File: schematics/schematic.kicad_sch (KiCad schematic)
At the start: 14 parts, among them J2 Conn_01x02, Q1 BPW40, U1 L293D, U2 ESP32-S3-DevKitC, U3 L7805

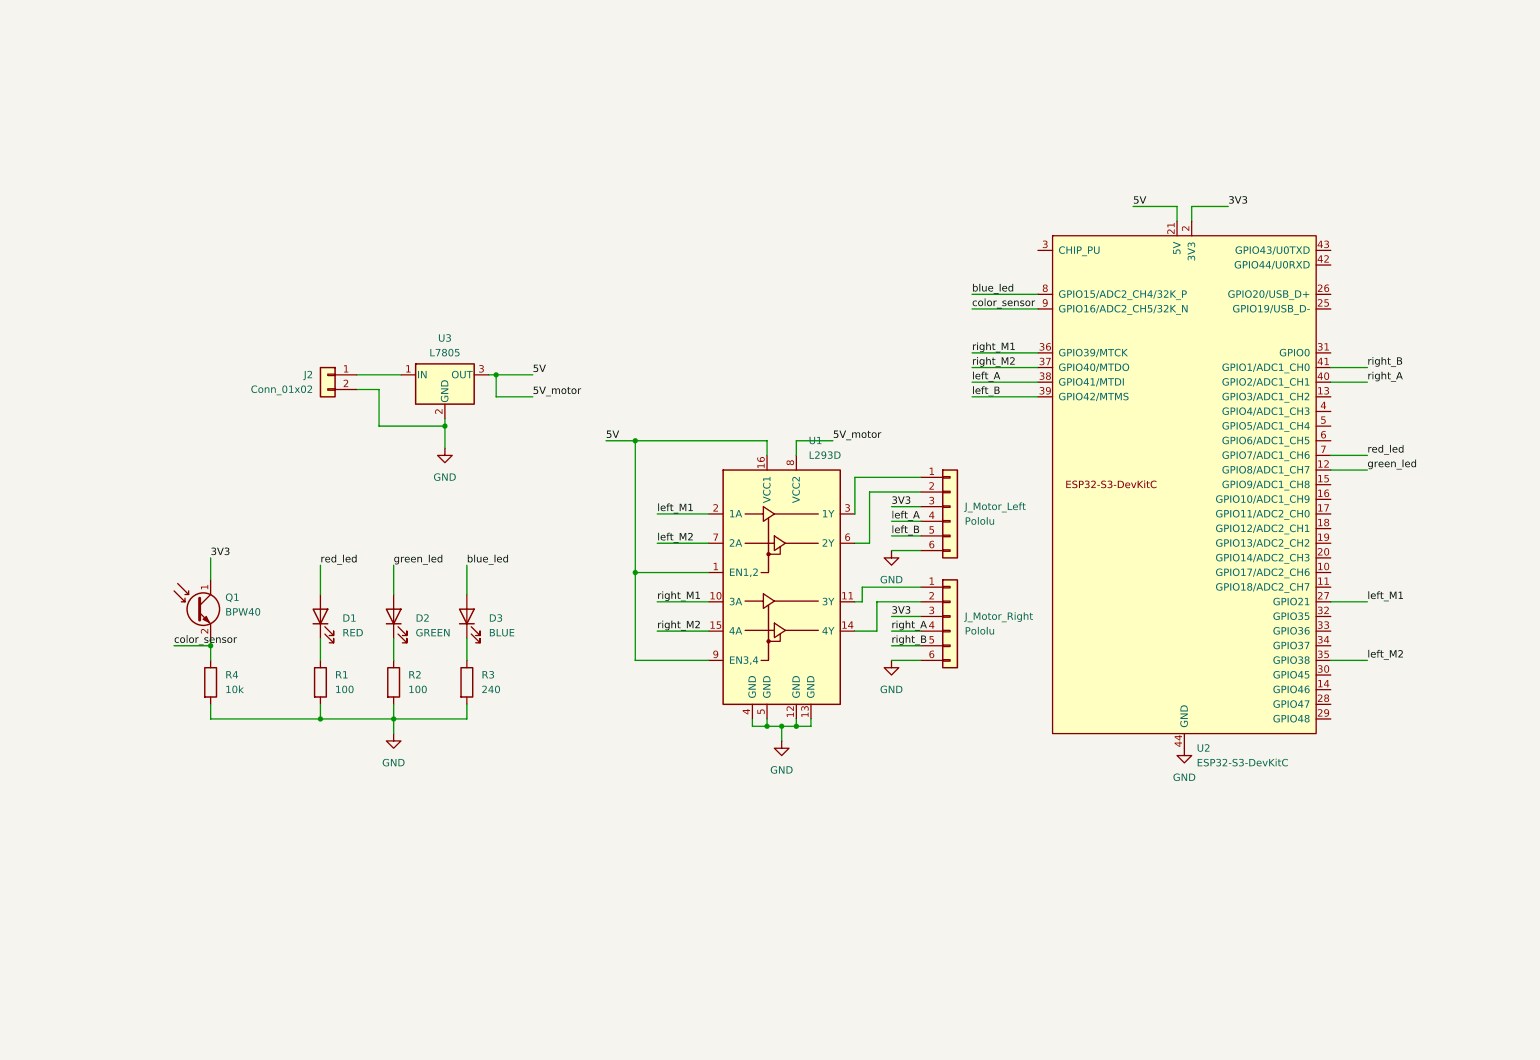
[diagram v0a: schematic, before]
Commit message: schematic update: almost done
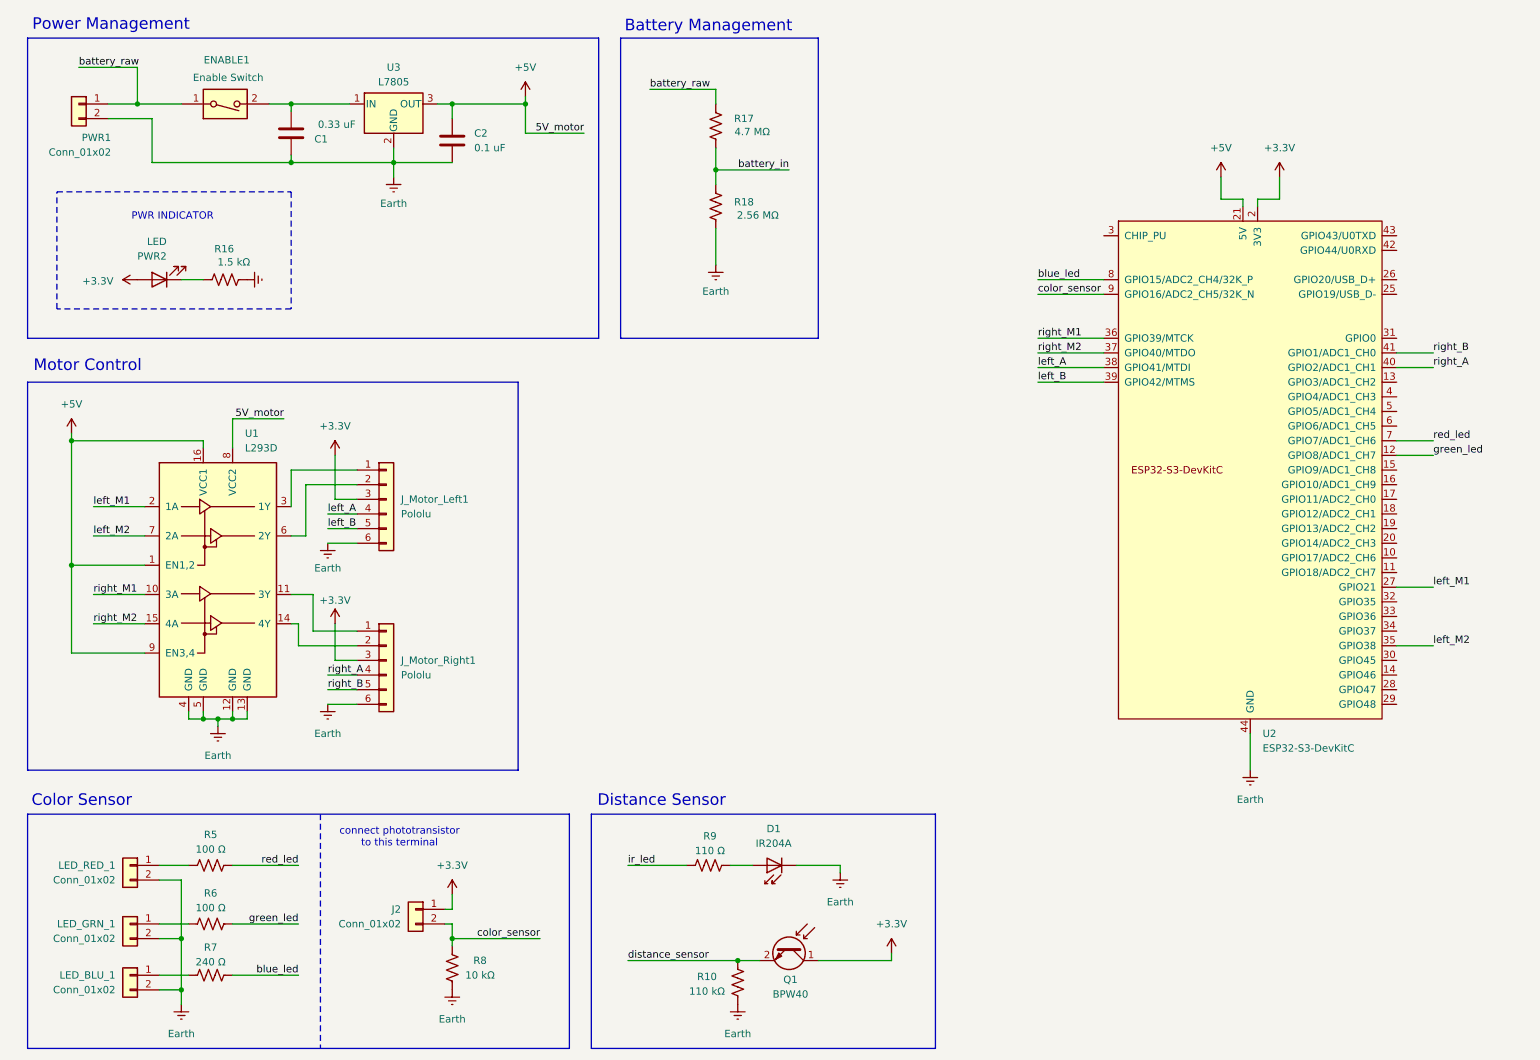
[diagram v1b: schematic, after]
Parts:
- removed D1: RED, symbol Device:LED
- removed D2: GREEN, symbol Device:LED
- removed D3: BLUE, symbol Device:LED
- removed R1, R2: 100, symbol Device:R
- removed R3: 240, symbol Device:R
- removed R4: 10k, symbol Device:R
- added C1: 0.33 uF, symbol TR3_V1:C
- added C2: 0.1 uF, symbol TR3_V1:C
- added D1: IR204A, LED_THT:LED_D3.0mm_IRBlack, symbol LED:IR204A
- added ENABLE1: Enable Switch, TR3_V1:SW_DS04-254-2-01BK-SMT, symbol TR3_V1:SW_DIP_x01
- added J2, LED_BLU_1, LED_GRN_1, LED_RED_1: Conn_01x02, symbol Connector_Generic:Conn_01x02
- added PWR2: LED, TR3_V1:150080RS75000_WRE, symbol TR3_V1:LED
- added R10: 110 kΩ, symbol TR3_V1:R_US
- added R16: 1.5 kΩ, Resistor_SMD:R_0603_1608Metric_Pad0.98x0.95mm_HandSolder, symbol TR3_V1:R_US
- added R17: 4.7 MΩ, Resistor_SMD:R_0603_1608Metric_Pad0.98x0.95mm_HandSolder, symbol TR3_V1:R_US
- added R18: 2.56 MΩ, Resistor_SMD:R_0603_1608Metric_Pad0.98x0.95mm_HandSolder, symbol TR3_V1:R_US
- added R5, R6: 100 Ω, symbol TR3_V1:R_US
- added R7: 240 Ω, symbol TR3_V1:R_US
- added R8: 10 kΩ, symbol TR3_V1:R_US
- added R9: 110 Ω, symbol TR3_V1:R_US
- U2: footprint PCM_Espressif:ESP32-S3-DevKitC -> footprints_pretty:XCVR_ESP32-S3-DEVKITC-1-N8R2
- renumbered J_Motor_Left to J_Motor_Left1, J_Motor_Right to J_Motor_Right1, J2 to PWR1
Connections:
- net blue_led: now also R7.2
- net color_sensor: now also J2.2 (Pin_2), R8.2; no longer Q1.2 (E)
- net green_led: now also R6.2
- net red_led: now also R5.2
- net at U3.1 (IN): now also C1.2, ENABLE1.2; no longer PWR1.1 (Pin_1)
- net 3V3 renamed +3.3V
- net +3.3V: now also J2.1 (Pin_1), PWR2.2 (A)
- net 5V renamed +5V
- net +5V: now also C2.1
- net GND renamed Earth
- net Earth: now also C1.1, C2.2, D1.1 (K), LED_BLU_1.2 (Pin_2), LED_GRN_1.2 (Pin_2), LED_RED_1.2 (Pin_2), R10.1, R16.2, R18.1, R8.1
- new net: LED_GRN_1.1 (Pin_1), R6.1
- new net: D1.2 (A), R9.2
- new net: LED_RED_1.1 (Pin_1), R5.1
- new net: PWR2.1 (K), R16.1
- new net: LED_BLU_1.1 (Pin_1), R7.1
- new net battery_in: R17.1, R18.2
- new net battery_raw: ENABLE1.1, PWR1.1 (Pin_1), R17.2
- new net distance_sensor: Q1.2 (E), R10.2
- new net ir_led: R9.1
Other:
- note added: "Battery Management"
- note added: "Color Sensor"
- note added: "Distance Sensor"
- note added: "Motor Control"
- note added: "PWR INDICATOR"
- note added: "Power Management"
- note added: "connect phototransistor to this terminal"
- moved on the sheet: J_Motor_Left1, J_Motor_Right1, PWR1, U1, U2, U3

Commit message: schematic done
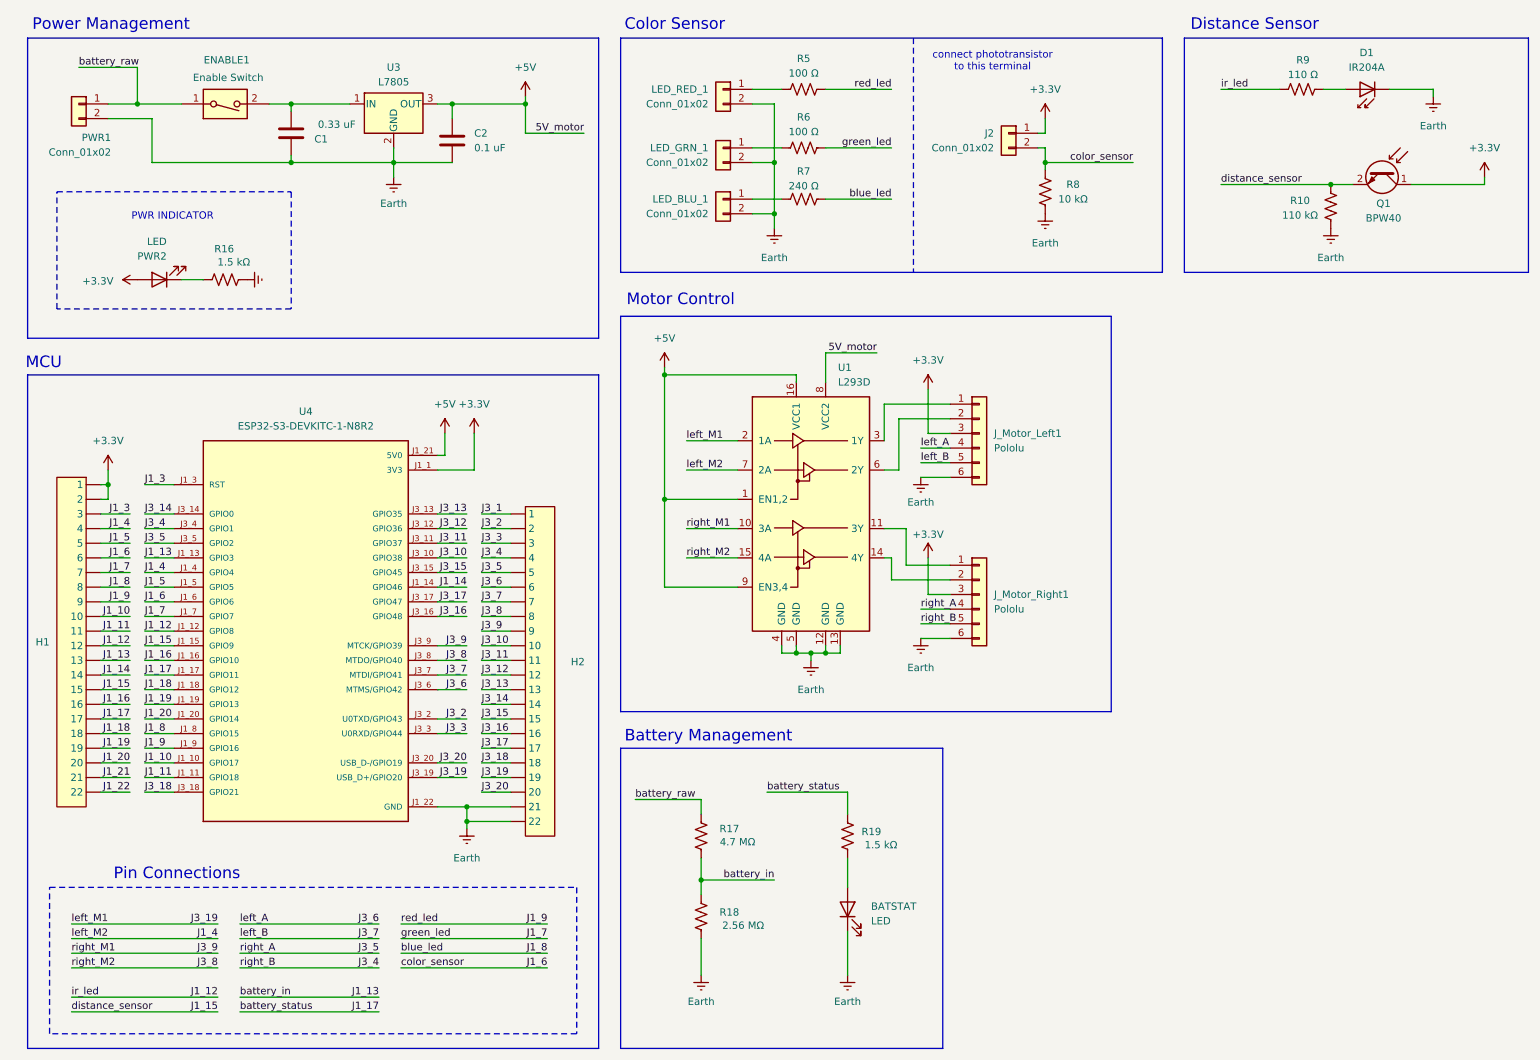
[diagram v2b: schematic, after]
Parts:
- removed U2: ESP32-S3-DevKitC, footprints_pretty:XCVR_ESP32-S3-DEVKITC-1-N8R2, symbol PCM_Espressif:ESP32-S3-DevKitC
- added BATSTAT: LED, LED_SMD:LED_0201_0603Metric, symbol TR3_V1:LED
- added H1, H2: (no value), symbol schematic:22_pin_header
- added R19: 1.5 kΩ, Resistor_SMD:R_0201_0603Metric, symbol TR3_V1:R_US
- added U4: ESP32-S3-DEVKITC-1-N8R2, ESP32-S3-DEVKITC-1-N8R2:XCVR_ESP32-S3-DEVKITC-1-N8R2, symbol ESP32-S3-DEVKITC-1-N8R2:ESP32-S3-DEVKITC-1-N8R2
- C1, C2: footprint (none) -> Capacitor_SMD:C_0201_0603Metric
- PWR2: footprint TR3_V1:150080RS75000_WRE -> LED_SMD:LED_0201_0603Metric
- R10, R5, R6, R7, R8, R9: footprint (none) -> Resistor_SMD:R_0201_0603Metric
- R16: footprint Resistor_SMD:R_0603_1608Metric_Pad0.98x0.95mm_HandSolder -> Resistor_SMD:R_0201_0603Metric
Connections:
- net +3.3V: now also H1. (22), U4.J1_1 (3V3), U4.J1_2 (3V3)
- net +5V: now also U4.J1_21 (5V0)
- net Earth: now also BATSTAT.1 (K), H2. (22), U4.J1_22 (GND), U4.J3_1 (GND), U4.J3_21 (GND), U4.J3_22 (GND)
- net battery_in renamed J1_13
- net J1_13: now also H1. (22), U4.J1_13 (GPIO3)
- net blue_led renamed J1_8
- net J1_8: now also H1. (22), U4.J1_8 (GPIO15)
- net color_sensor renamed J1_6
- net J1_6: now also H1. (22), U4.J1_6 (GPIO6)
- net distance_sensor renamed J1_15
- net J1_15: now also H1. (22), U4.J1_15 (GPIO9)
- net green_led renamed J1_7
- net J1_7: now also H1. (22), U4.J1_7 (GPIO7)
- net ir_led renamed J1_12
- net J1_12: now also H1. (22), U4.J1_12 (GPIO8)
- net left_A renamed J3_6
- net J3_6: now also H2. (22), U4.J3_6 (MTMS/GPIO42)
- net left_B renamed J3_7
- net J3_7: now also H2. (22), U4.J3_7 (MTDI/GPIO41)
- net left_M1 renamed J3_19
- net J3_19: now also H2. (22), U4.J3_19 (USB_D+/GPIO20)
- net left_M2 renamed J1_4
- net J1_4: now also H1. (22), U4.J1_4 (GPIO4)
- net red_led renamed J1_9
- net J1_9: now also H1. (22), U4.J1_9 (GPIO16)
- net right_A renamed J3_5
- net J3_5: now also H2. (22), U4.J3_5 (GPIO2)
- net right_B renamed J3_4
- net J3_4: now also H2. (22), U4.J3_4 (GPIO1)
- net right_M1 renamed J3_9
- net J3_9: now also H2. (22), U4.J3_9 (MTCK/GPIO39)
- net right_M2 renamed J3_8
- net J3_8: now also H2. (22), U4.J3_8 (MTDO/GPIO40)
- new net: BATSTAT.2 (A), R19.2
- new net J1_10: H1. (22), U4.J1_10 (GPIO17)
- new net J1_11: H1. (22), U4.J1_11 (GPIO18)
- new net J1_14: H1. (22), U4.J1_14 (GPIO46)
- new net J1_16: H1. (22), U4.J1_16 (GPIO10)
- new net J1_17: H1. (22), R19.1, U4.J1_17 (GPIO11)
- new net J1_18: H1. (22), U4.J1_18 (GPIO12)
- new net J1_19: H1. (22), U4.J1_19 (GPIO13)
- new net J1_20: H1. (22), U4.J1_20 (GPIO14)
- new net J1_21: H1. (22)
- new net J1_22: H1. (22)
- new net J1_3: H1. (22), U4.J1_3 (RST)
- new net J1_5: H1. (22), U4.J1_5 (GPIO5)
- new net J3_1: H2. (22)
- new net J3_10: H2. (22), U4.J3_10 (GPIO38)
- new net J3_11: H2. (22), U4.J3_11 (GPIO37)
- new net J3_12: H2. (22), U4.J3_12 (GPIO36)
- new net J3_13: H2. (22), U4.J3_13 (GPIO35)
- new net J3_14: H2. (22), U4.J3_14 (GPIO0)
- new net J3_15: H2. (22), U4.J3_15 (GPIO45)
- new net J3_16: H2. (22), U4.J3_16 (GPIO48)
- new net J3_17: H2. (22), U4.J3_17 (GPIO47)
- new net J3_18: H2. (22), U4.J3_18 (GPIO21)
- new net J3_2: H2. (22), U4.J3_2 (U0TXD/GPIO43)
- new net J3_20: H2. (22), U4.J3_20 (USB_D-/GPIO19)
- new net J3_3: H2. (22), U4.J3_3 (U0RXD/GPIO44)
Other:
- note added: "MCU"
- note added: "Pin Connections"
- moved on the sheet: D1, J2, J_Motor_Left1, J_Motor_Right1, LED_BLU_1, LED_GRN_1, LED_RED_1, Q1, R10, R17, R18, R5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
